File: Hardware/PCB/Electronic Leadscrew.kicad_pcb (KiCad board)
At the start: 2 copper layers, 61.8 x 130 mm, 26 parts, among them J101 DISPLAY, J102 ENCODER, J103 STEPPER DRIVER, Q101 SI2302, Q102 SI2302, Q103 SI2302, U101 PI PICO, U102 TPT480L1-SO1R, U103 SDB628

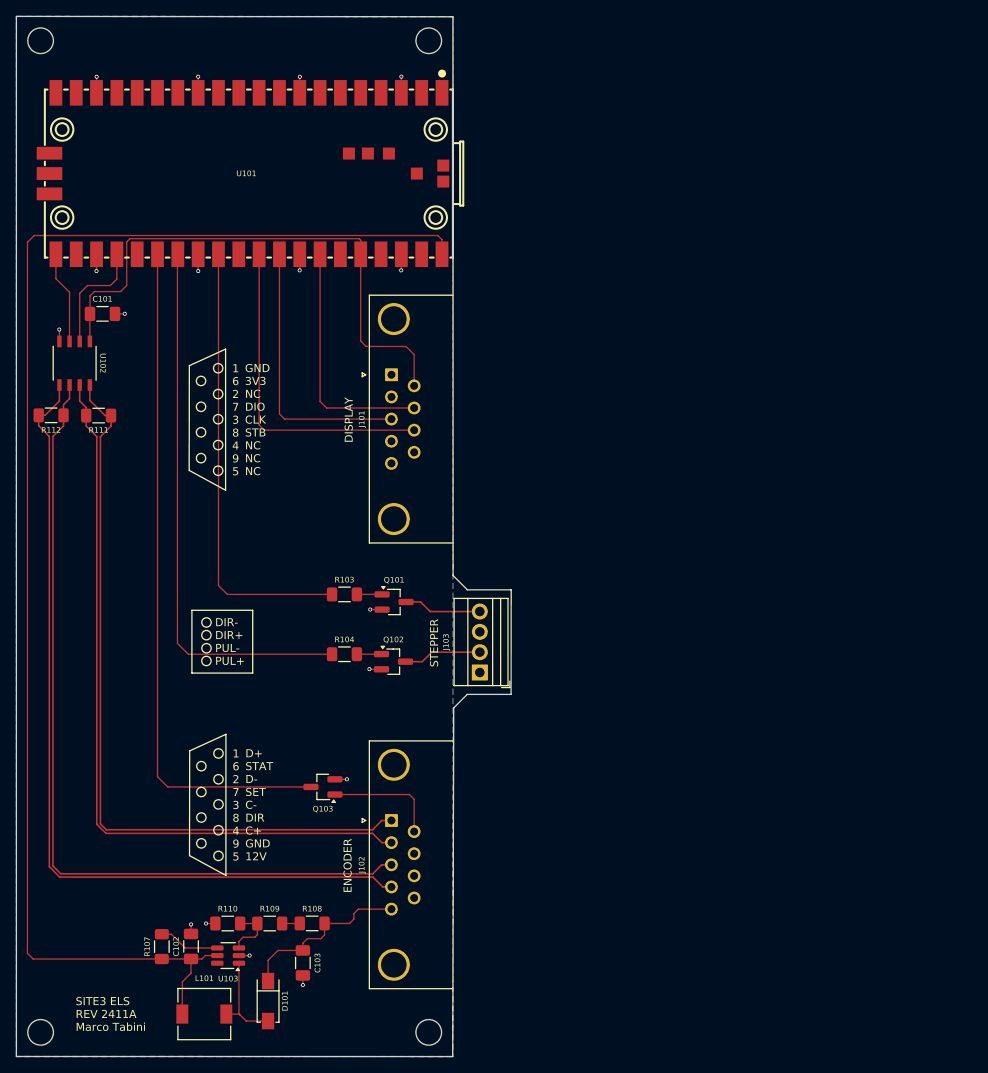
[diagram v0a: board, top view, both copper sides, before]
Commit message: Update PCB
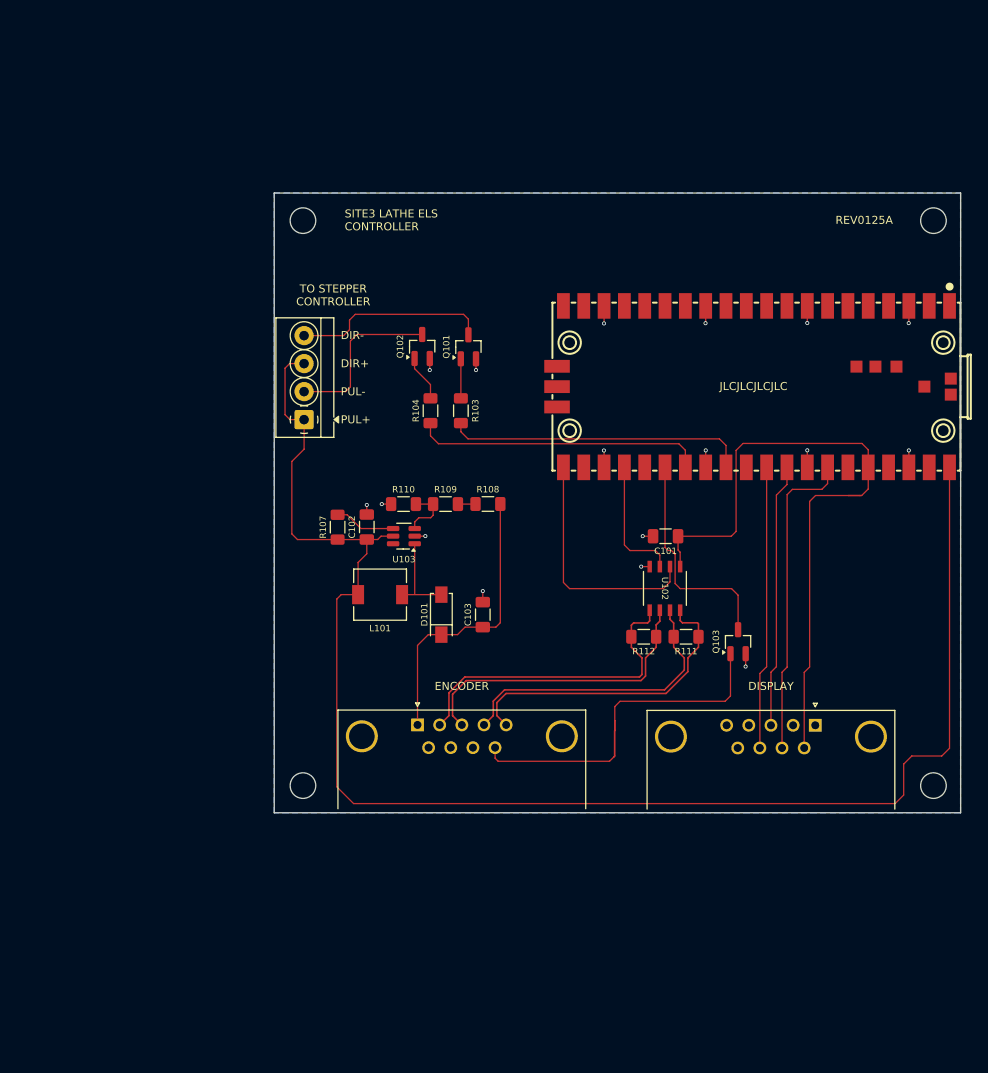
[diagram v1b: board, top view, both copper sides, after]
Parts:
- removed the REF** at (84.7, 43.0)
- removed the REF** at (133.3, 43.0)
- removed the REF** at (84.7, 167.0)
- removed the REF** at (133.3, 167.0)
- added REF**: MountingHole_3.2mm_M3, MountingHole:MountingHole_3.2mm_M3, F.Cu at (117.5, 65.5)
- added REF**: MountingHole_3.2mm_M3, MountingHole:MountingHole_3.2mm_M3, F.Cu at (196.3, 65.5)
- added REF**: MountingHole_3.2mm_M3, MountingHole:MountingHole_3.2mm_M3, F.Cu at (196.3, 136.1)
- added REF**: MountingHole_3.2mm_M3, MountingHole:MountingHole_3.2mm_M3, F.Cu at (117.5, 136.1)
- J101: footprint Connector_Dsub:DSUB-9_Female_Horizontal_P2.77x2.84mm_EdgePinOffset4.94mm_Housed_MountingHolesOffset7.48mm -> Connector_Dsub:DSUB-9_Female_Horizontal_P2.77x2.84mm_EdgePinOffset7.70mm_Housed_MountingHolesOffset9.12mm
- J102: footprint Connector_Dsub:DSUB-9_Female_Horizontal_P2.77x2.84mm_EdgePinOffset4.94mm_Housed_MountingHolesOffset7.48mm -> Connector_Dsub:DSUB-9_Male_Horizontal_P2.77x2.84mm_EdgePinOffset7.70mm_Housed_MountingHolesOffset9.12mm
- J103: footprint TerminalBlock:TerminalBlock_Xinya_XY308-2.54-4P_1x04_P2.54mm_Horizontal -> TerminalBlock_4Ucon:TerminalBlock_4Ucon_1x04_P3.50mm_Horizontal
- moved R112 79.1 mm to (160.1, 117.5)
- moved U102 79.0 mm to (162.8, 111.5)
- moved R111 78.5 mm to (165.4, 117.5)
- moved C101 75.7 mm to (162.9, 104.9), turned to 180 degrees
- moved U101 68.8 mm to (173.9, 86.2)
- moved J101 68.8 mm to (181.6, 128.6), turned to 0 degrees
- moved C102 56.8 mm to (125.5, 103.8)
- moved R107 56.8 mm to (121.9, 103.8)
- moved R108 56.8 mm to (140.7, 100.9)
- moved L101 56.8 mm to (127.2, 112.2)
- moved R109 56.8 mm to (135.4, 100.9)
- moved R110 56.8 mm to (130.1, 100.9)
- moved U103 56.8 mm to (130.2, 104.9)
- moved Q103 55.0 mm to (171.9, 118.1), turned to 90 degrees
- moved D101 52.9 mm to (134.8, 114.7), turned to 90 degrees
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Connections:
- J101 pad 2: /NC -> unconnected-(J101-Pad2)
- J102 pad 1: /ENC_DAT+ -> +12V
- J102 pad 2: /ENC_DAT- -> /ENC_CLK+
- J102 pad 4: /ENC_CLK+ -> /ENC_DAT-
- J102 pad 5: +12V -> /ENC_DAT+
- J102 pad 6: /~{ENC_STAT} -> GND
- J102 pad 7: /ENC_SET -> GND
- J102 pad 8: /ENC_DIR -> GND
- J102 pad 9: GND -> /~{ENC_STAT}
- J103 pad 1: /STP_PUL+ -> +5V
- J103 pad 3: /STP_DIR+ -> +5V
- U101 pad 21: /ENC_CLK -> /ENC_DAT
- U101 pad 24: /ENC_DAT -> /ENC_CLK
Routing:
- net /ENC_CLK+: track 106.1 -> 40.1 mm
- net /ENC_CLK-: track 104.2 -> 38.3 mm
- net Net-(Q103-D): track 85.0 -> 28.1 mm
- net /ENC_DAT-: track 93.6 -> 37.2 mm
- net /ENC_DAT+: track 94.1 -> 39.0 mm
- net /~{ENC_STAT}: track 14.2 -> 47.8 mm
- net Net-(U101-GP21): track 68.5 -> 36.3 mm
- net Net-(U101-GP22): track 56.1 -> 37.7 mm
- net +5V: track 174.6 -> 190.5 mm
- net /ENC_DAT: track 14.5 -> 30.3 mm
- net /STP_DIR-: track 9.71 -> 24.5 mm
- net +3.3V: track 69.7 -> 84.3 mm
- net +12V: track 22.5 -> 36.3 mm
- net /STP_PUL-: track 9.78 -> 21.1 mm
- net /DIS_DIO: track 30.5 -> 39.6 mm
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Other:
- board size 61.8 x 130 mm -> 85.8 x 77.5 mm
- board text added: "+"
- board text added: "+12V"
- board text added: "-"
- board text added: "3V3"
- board text added: "CLK"
- board text added: "DAT"
- board text added: "DIO"
- board text added: "DIR+"
- board text added: "DIR-"
- board text added: "GND"
- board text added: "JLCJLCJLCJLC"
- board text added: "PUL+"
- board text added: "PUL-"
- board text added: "REV0125A"
- board text added: "SITE3 LATHE ELS CONTROLLER"
- board text added: "STB"
- board text added: "TO STEPPER CONTROLLER"
- board text added: "~{STAT}"
- board text removed: "1 6 2 7 3 8 4 9 5"
- board text removed: "D+ STAT D- SET C- DIR C+ GND 12V"
- board text removed: "DIR- DIR+ PUL- PUL+"
- board text removed: "GND 3V3 NC DIO CLK STB NC NC NC"
- board text removed: "SITE3 ELS REV 2411A Marco Tabini"
- board text removed: "STEPPER"
